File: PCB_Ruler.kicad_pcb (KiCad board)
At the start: 2 copper layers, 100.5 x 27 mm, 119 parts, among them Q1 SOT23-3, Q10 SOT89, Q11 SOT886, Q12 SOT963, Q13 SSOP-16, Q14 SSOP-8, Q15 SOT1113, Q16 SOT665, Q17 SO-8, Q18 QFNx24, Q19 QFPx100_0.5, Q2 SOT23-5, Q20 QFPx32, Q21 QFPx32_0.8, Q22 QFPx100, Q23 SOIC, Q24 TSOP-48, Q25 BGA_DDR4, Q26 BGA_10x, Q27 BGA_4x, Q28 QNFx20, Q29 QNFx40, Q3 SOT323, Q30 QNFx48, Q31 QNFx64, Q32 QFPx48, Q33 QFPx64, Q34 BGA_5, Q35 BGA_78x, Q36 BGA_4, Q37 BGA_6x, Q38 BGA_5x_1.27, Q39 BGA_15x_0.65, Q4 SOT353, Q40 QNFx32, Q41 QNFx12, Q42 SC-59, Q43 BGA_8, Q5 SOT553, Q6 DPAK, Q7 DP2AK, Q8 LFPAK, Q9 SOT223, U1 1.00, U10 5mm, U11 6mm, U12 7mm, U13 8mm, U14 9mm, U15 3_10in, U16 0_16in, U17 1_16in, U18 2_16in, U19 3_16in, U2 1.27, U20 0_10in, U21 1_10in, U22 2_10in, U3 2.00, U4 2.54, U5 0mm, U6 1mm, U7 2mm, U8 3mm, U9 4mm

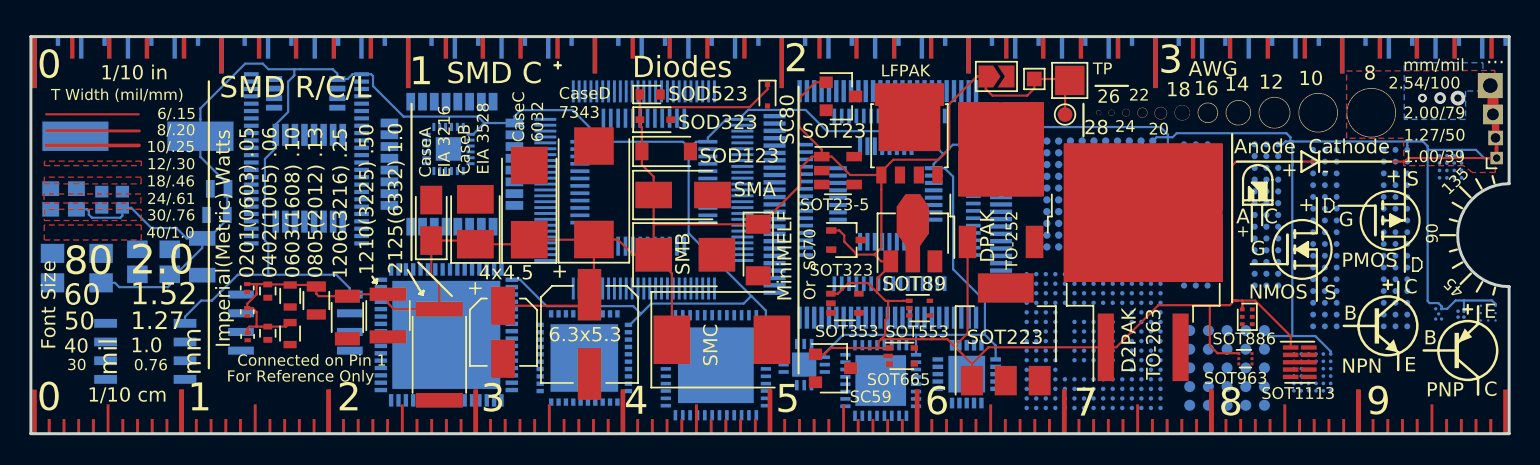
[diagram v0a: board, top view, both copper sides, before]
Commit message: Move a few things around
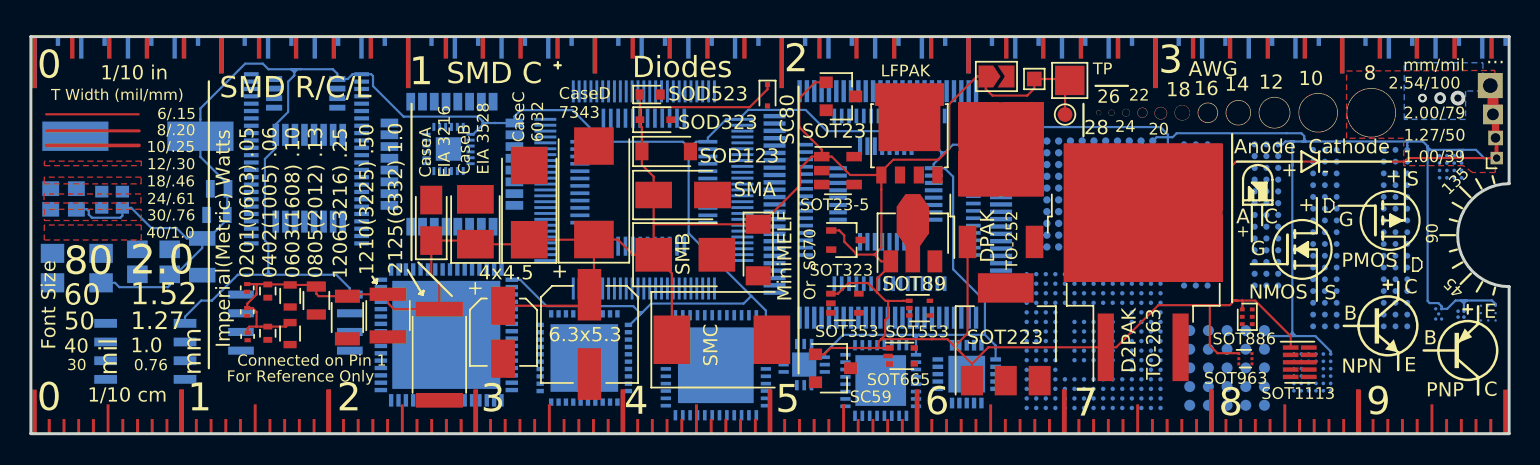
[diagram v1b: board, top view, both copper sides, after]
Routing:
- net /Pin1: track 506.8 -> 514.1 mm
